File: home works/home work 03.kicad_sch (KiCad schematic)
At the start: 0 parts

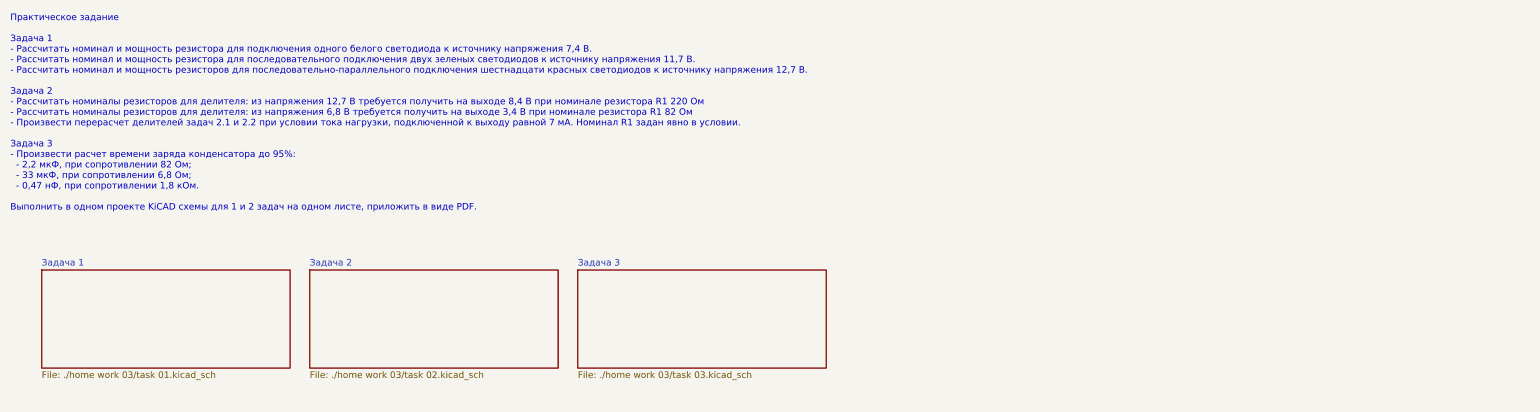
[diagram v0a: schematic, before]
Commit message: home works 3 and 4
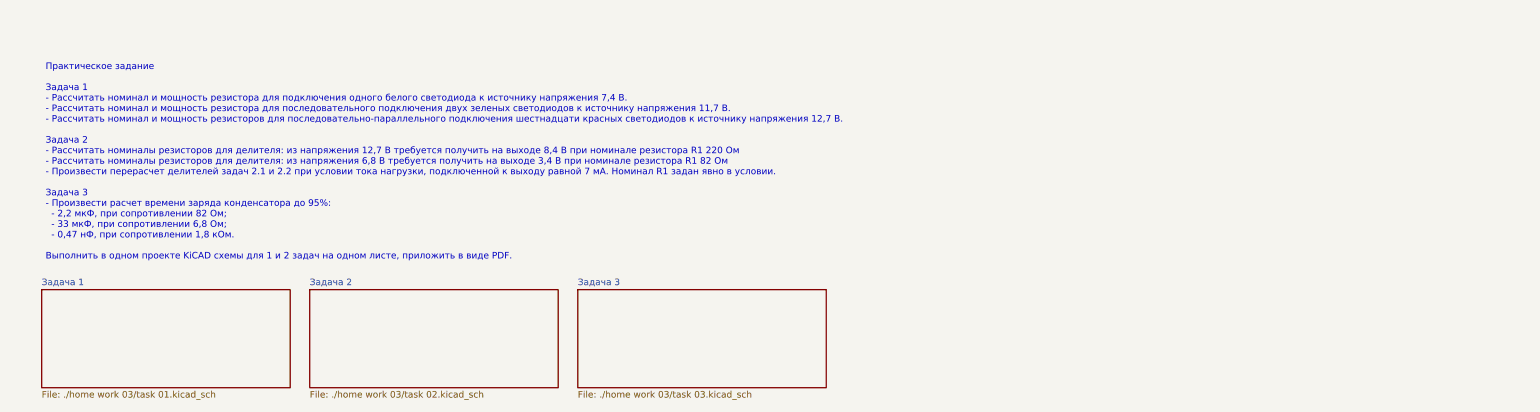
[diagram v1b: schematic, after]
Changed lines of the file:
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@@
 	(text "Практическое задание\n\nЗадача 1\n- Рассчитать номинал и мощность резистора для подключения одного белого светодиода к источнику напряжения 7,4 В.\n- Рассчитать номинал и мощность резистора для последовательного подключения двух зеленых светодиодов к источнику напряжения 11,7 В.\n- Рассчитать номинал и мощность резисторов для последовательно-параллельного подключения шестнадцати красных светодиодов к источнику напряжения 12,7 В.\n\nЗадача 2\n- Рассчитать номиналы резисторов для делителя: из напряжения 12,7 В требуется получить на выходе 8,4 В при номинале резистора R1 220 Ом\n- Рассчитать номиналы резисторов для делителя: из напряжения 6,8 В требуется получить на выходе 3,4 В при номинале резистора R1 82 Ом\n- Произвести перерасчет делителей задач 2.1 и 2.2 при условии тока нагрузки, подключенной к выходу равной 7 мА. Номинал R1 задан явно в условии.\n\nЗадача 3 \n- Произвести расчет времени заряда конденсатора до 95%:\n  - 2,2 мкФ, при сопротивлении 82 Ом;\n  - 33 мкФ, при сопротивлении 6,8 Ом;\n  - 0,47 нФ, при сопротивлении 1,8 кОм.\n\nВыполнить в одном проекте KiCAD схемы для 1 и 2 задач на одном листе, приложить в виде PDF.\n\n"
 		(exclude_from_sim no)
-		(at 18.034 36.576 0)
+		(at 24.892 25.908 0)
 		(effects
 			(font
 				(size 1.27 1.27)
 			)
-			(justify left)
+			(justify left top)
 		)
 	)
 	(sheet
-		(at 24.13 66.04)
+		(at 24.13 69.85)
 		(size 48.26 19.05)
 		(fields_autoplaced yes)
@@
 		)
 		(property "Sheetname" "Задача 1"
-			(at 24.13 65.3284 0)
+			(at 24.13 69.1384 0)
 			(effects
 				(font
@@
 		)
 		(property "Sheetfile" "./home work 03/task 01.kicad_sch"
-			(at 24.13 85.6746 0)
+			(at 24.13 89.4846 0)
 			(effects
 				(font
@@
 	)
 	(sheet
-		(at 128.27 66.04)
+		(at 128.27 69.85)
 		(size 48.26 19.05)
 		(fields_autoplaced yes)
@@
 		)
 		(property "Sheetname" "Задача 3"
-			(at 128.27 65.3284 0)
+			(at 128.27 69.1384 0)
 			(effects
 				(font
@@
 		)
 		(property "Sheetfile" "./home work 03/task 03.kicad_sch"
-			(at 128.27 85.6746 0)
+			(at 128.27 89.4846 0)
 			(effects
 				(font
@@
 	)
 	(sheet
-		(at 76.2 66.04)
+		(at 76.2 69.85)
 		(size 48.26 19.05)
 		(fields_autoplaced yes)
@@
 		)
 		(property "Sheetname" "Задача 2"
-			(at 76.2 65.3284 0)
+			(at 76.2 69.1384 0)
 			(effects
 				(font
@@
 		)
 		(property "Sheetfile" "./home work 03/task 02.kicad_sch"
-			(at 76.2 85.6746 0)
+			(at 76.2 89.4846 0)
 			(effects
 				(font
